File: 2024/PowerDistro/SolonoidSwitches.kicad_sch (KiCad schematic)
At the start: 4 parts, among them J13 Screw_Terminal_01x02, J14 Screw_Terminal_01x02, J15 Screw_Terminal_01x02, J16 Screw_Terminal_01x02

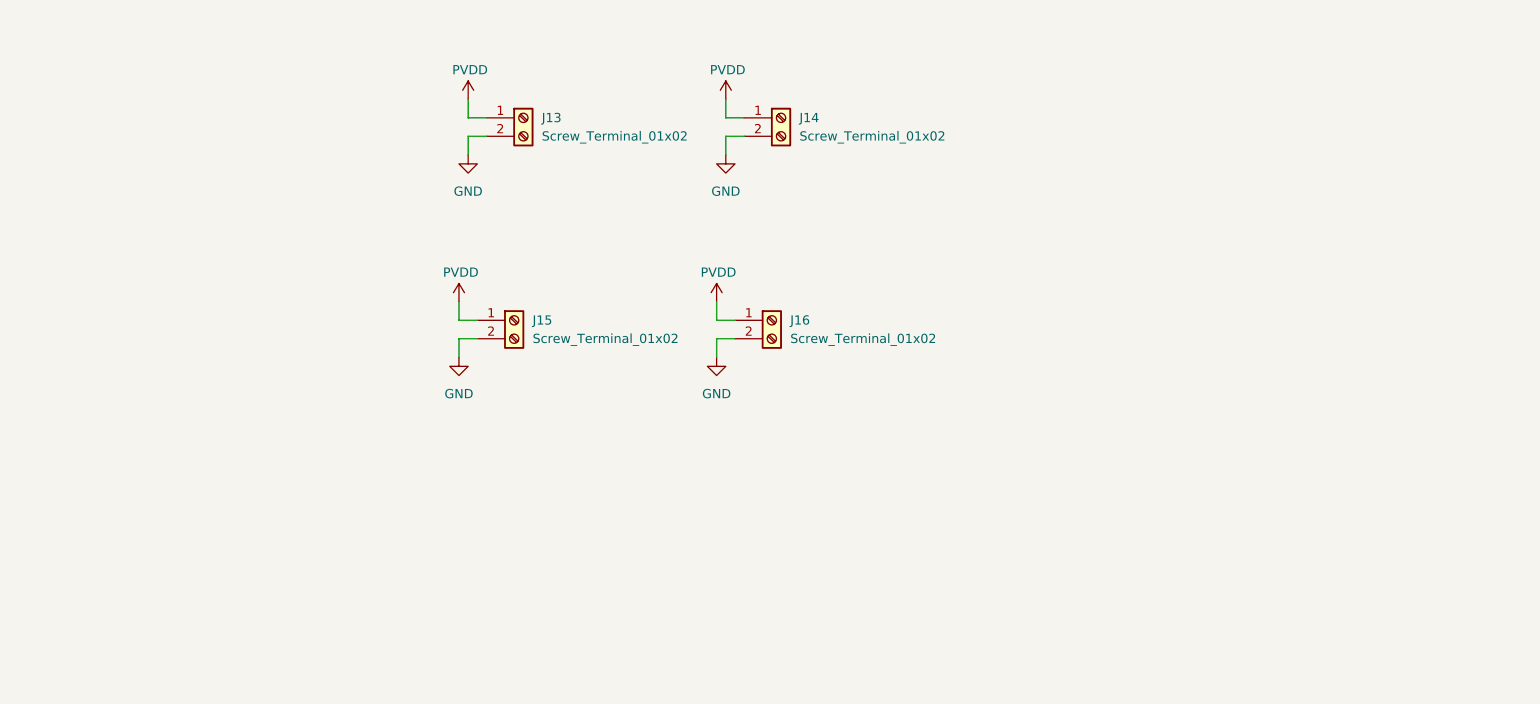
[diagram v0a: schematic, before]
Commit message: Release
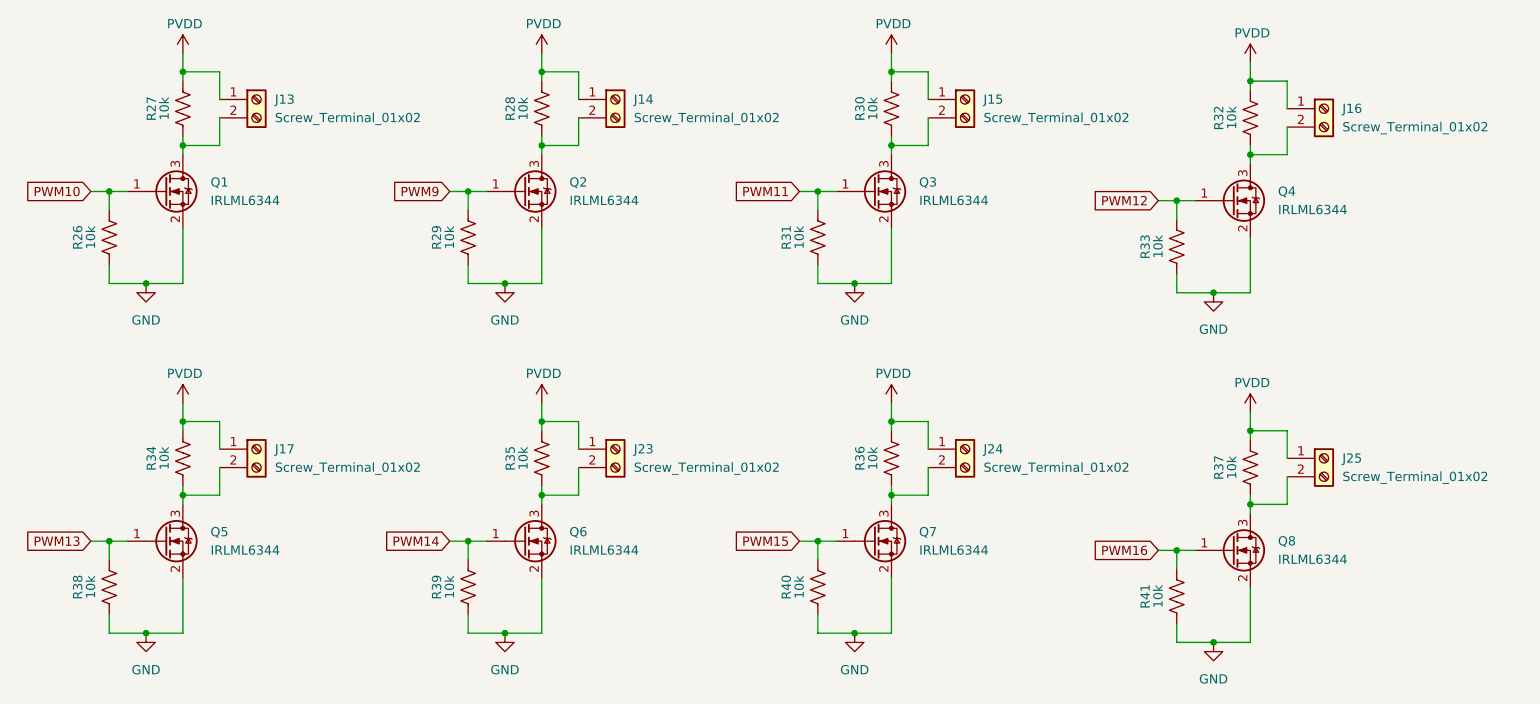
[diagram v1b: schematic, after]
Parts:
- added J17, J23, J24, J25: Screw_Terminal_01x02, PowerDistroFootprints:691321100002, symbol Connector:Screw_Terminal_01x02
- added Q1, Q2, Q3, Q4, Q5, Q6, Q7, Q8: IRLML6344, Package_TO_SOT_SMD:SOT-23, symbol Transistor_FET:IRLML6244
- added R26, R27, R28, R29, R30, R31, R32, R33, R34, R35, R36, R37, R38, R39, R40, R41: 10k, Resistor_SMD:R_0603_1608Metric, symbol Device:R_US
- J13, J14, J15, J16: footprint PowerDistroFootprints:691311500102 -> PowerDistroFootprints:691321100002
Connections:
- net GND: now also Q1.2 (S), Q2.2 (S), Q3.2 (S), Q4.2 (S), Q5.2 (S), Q6.2 (S), Q7.2 (S), Q8.2 (S), R26.2, R29.2, R31.2, R33.2, R38.2, R39.2, R40.2, R41.2; no longer J13.2 (Pin_2), J14.2 (Pin_2), J15.2 (Pin_2), J16.2 (Pin_2)
- net PVDD: now also J17.1 (Pin_1), J23.1 (Pin_1), J24.1 (Pin_1), J25.1 (Pin_1), R27.1, R28.1, R30.1, R32.1, R34.1, R35.1, R36.1, R37.1
- new net: J24.2 (Pin_2), Q7.3 (D), R36.2
- new net: J17.2 (Pin_2), Q5.3 (D), R34.2
- new net: J25.2 (Pin_2), Q8.3 (D), R37.2
- new net: J23.2 (Pin_2), Q6.3 (D), R35.2
- new net: J15.2 (Pin_2), Q3.3 (D), R30.2
- new net: J14.2 (Pin_2), Q2.3 (D), R28.2
- new net: J13.2 (Pin_2), Q1.3 (D), R27.2
- new net: J16.2 (Pin_2), Q4.3 (D), R32.2
- new net PWM10: Q1.1 (G), R26.1
- new net PWM11: Q3.1 (G), R31.1
- new net PWM12: Q4.1 (G), R33.1
- new net PWM13: Q5.1 (G), R38.1
- new net PWM14: Q6.1 (G), R39.1
- new net PWM15: Q7.1 (G), R40.1
- new net PWM16: Q8.1 (G), R41.1
- new net PWM9: Q2.1 (G), R29.1
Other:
- moved on the sheet: J13
